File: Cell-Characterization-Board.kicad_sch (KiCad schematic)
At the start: 1 part, among them U1 ESP32-S3-WROOM-1

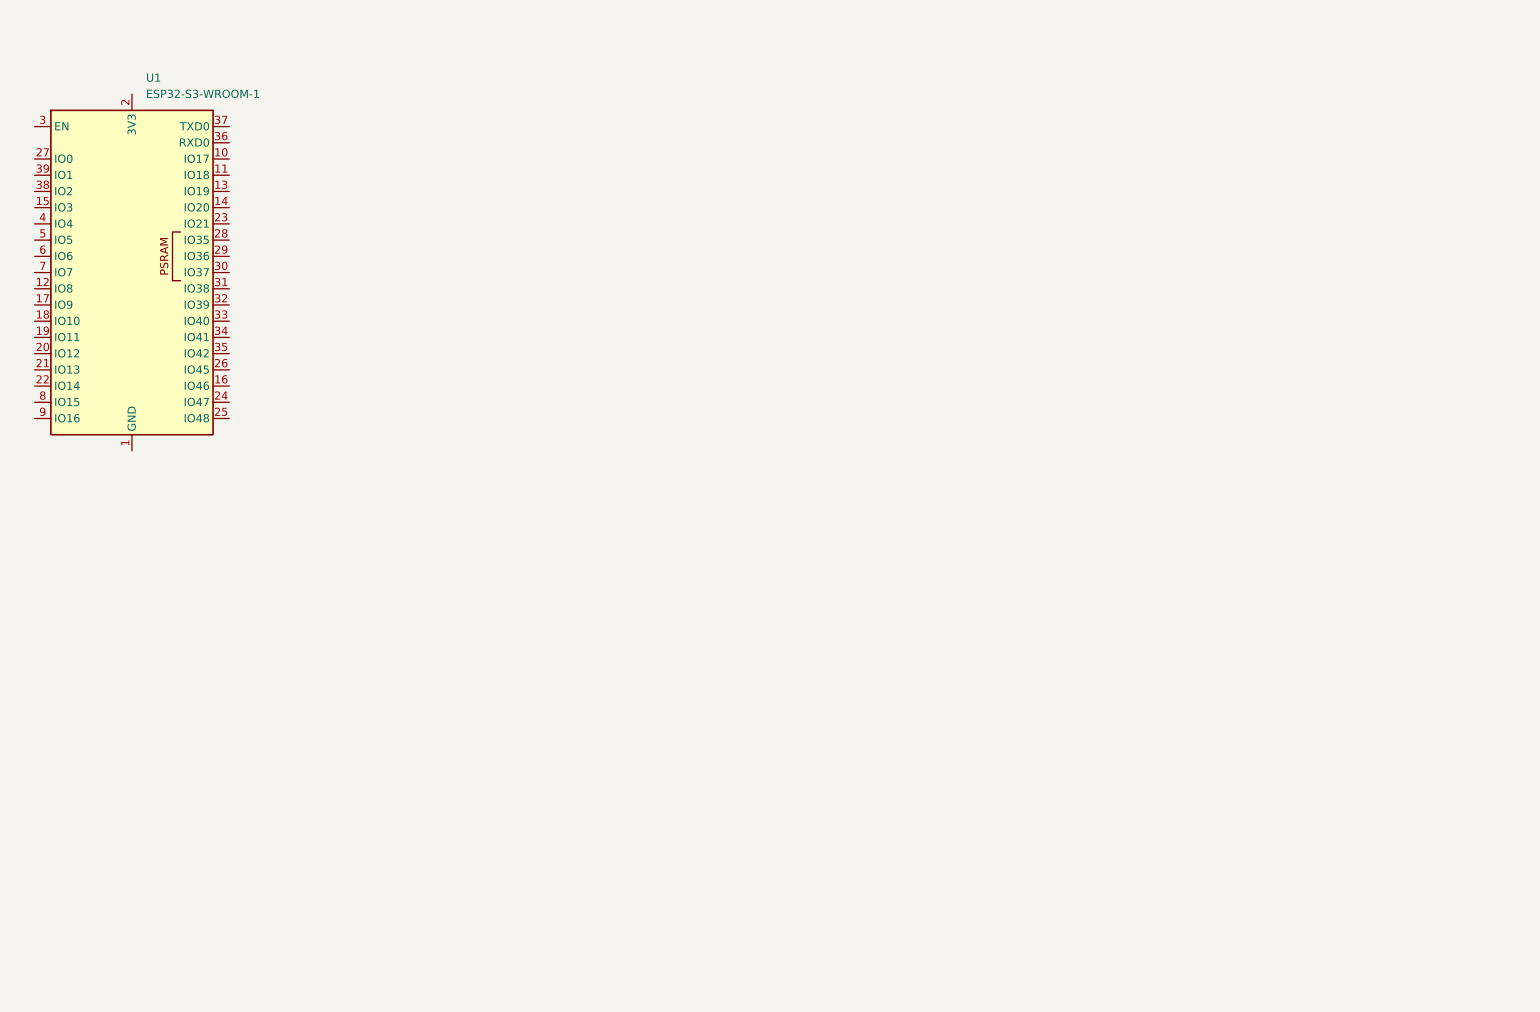
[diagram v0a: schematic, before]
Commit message: 🤪
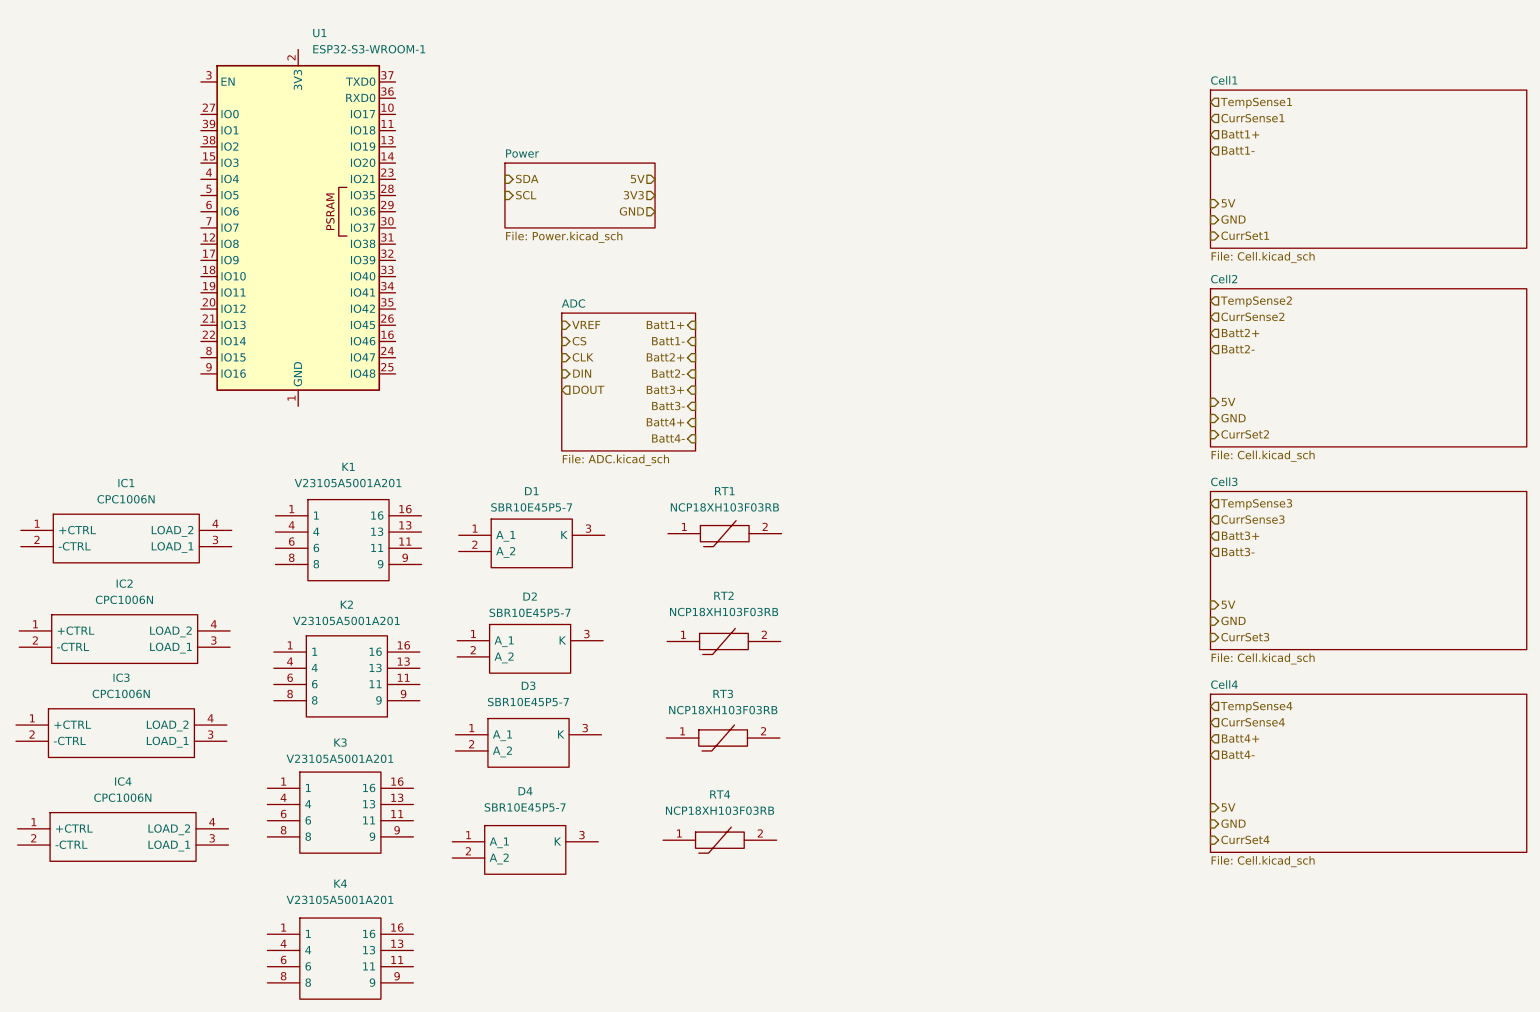
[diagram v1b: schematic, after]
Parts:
- added D1, D2, D3, D4: SBR10E45P5-7, SBR10E45P57, symbol SBR10E45P5-7:SBR10E45P5-7
- added IC1, IC2, IC3, IC4: CPC1006N, SOP254P610X216-4N, symbol CPC1006N:CPC1006N
- added K1, K2, K3, K4: V23105A5001A201, V23105A5001A201, symbol V23105A5001A201:V23105A5001A201
- added RT1, RT2, RT3, RT4: NCP18XH103F03RB, THRMC1608X95N, symbol NCP18XH103F03RB:NCP18XH103F03RB
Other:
- added sheet ADC (ADC.kicad_sch)
- added sheet Cell1 (Cell.kicad_sch)
- added sheet Cell2 (Cell.kicad_sch)
- added sheet Cell3 (Cell.kicad_sch)
- added sheet Cell4 (Cell.kicad_sch)
- added sheet Power (Power.kicad_sch)
- moved on the sheet: U1

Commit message: Updated main schematic
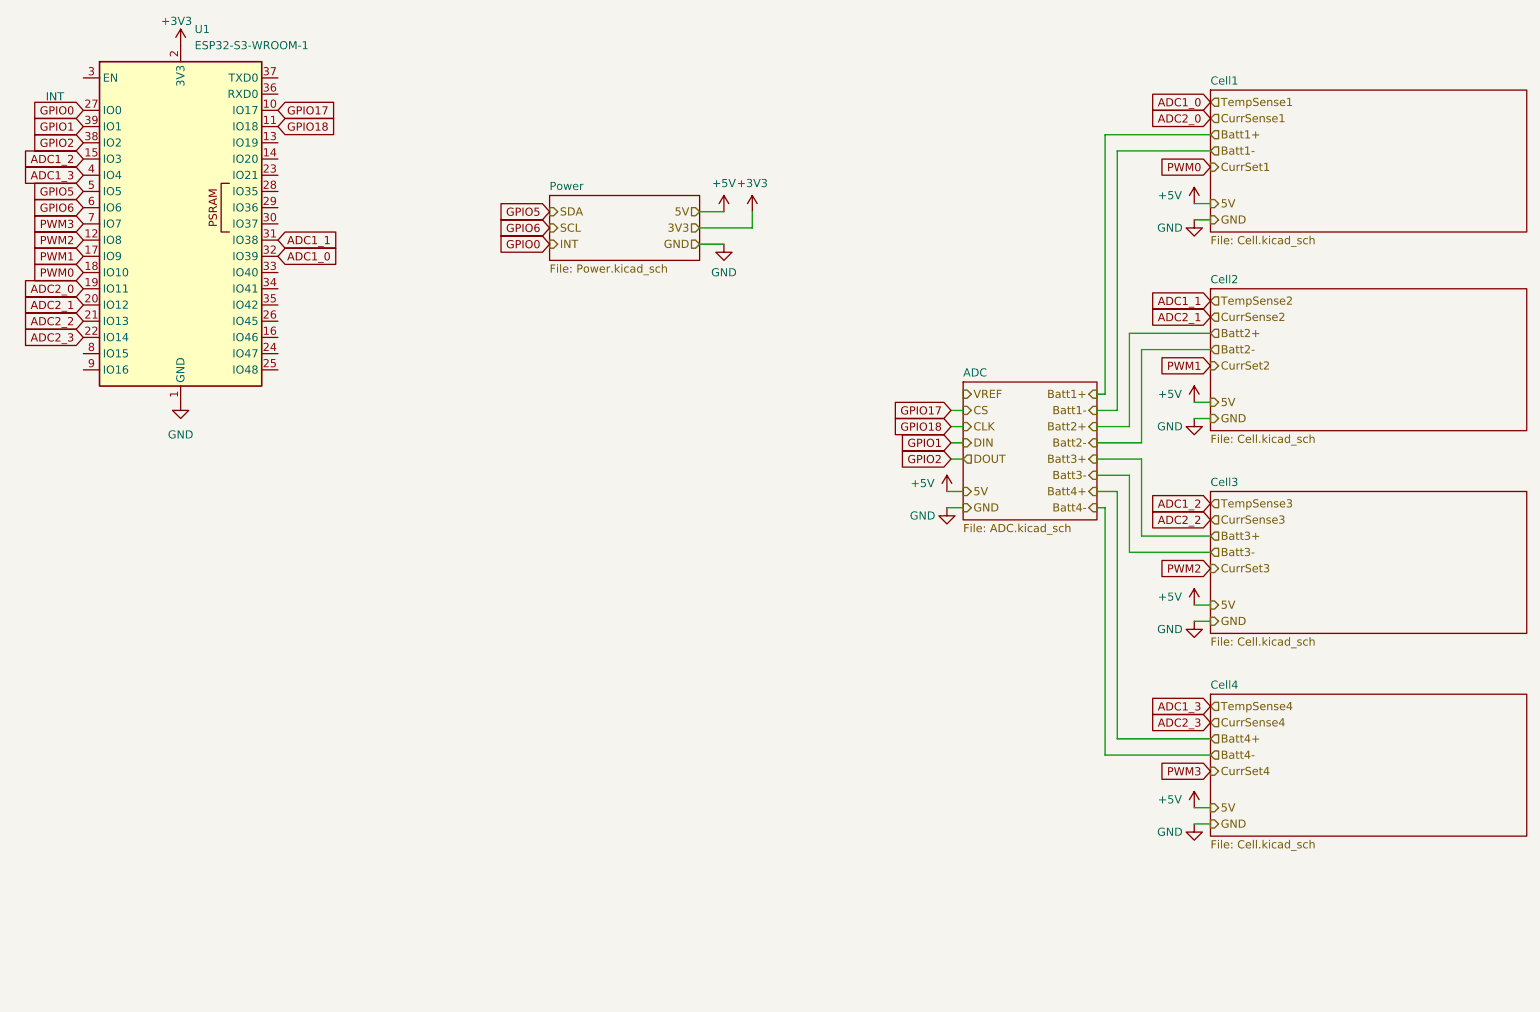
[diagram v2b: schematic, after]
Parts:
- removed D1, D2, D3, D4: SBR10E45P5-7, SBR10E45P57, symbol SBR10E45P5-7:SBR10E45P5-7
- removed IC1, IC2, IC3, IC4: CPC1006N, SOP254P610X216-4N, symbol CPC1006N:CPC1006N
- removed K1, K2, K3, K4: V23105A5001A201, V23105A5001A201, symbol V23105A5001A201:V23105A5001A201
- removed RT1, RT2, RT3, RT4: NCP18XH103F03RB, THRMC1608X95N, symbol NCP18XH103F03RB:NCP18XH103F03RB
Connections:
- net GND: now also U1.1 (GND), U1.40 (GND), U1.41 (GND)
- net GPIO17: now reaches U1.10 (IO17)
- net GPIO18: now reaches U1.11 (IO18)
- net PWM2: now reaches U1.12 (IO8)
- net ADC1_2: now reaches U1.15 (IO3)
- net PWM1: now reaches U1.17 (IO9)
- net PWM0: now reaches U1.18 (IO10)
- net ADC2_0: now reaches U1.19 (IO11)
- net +3V3: now reaches U1.2 (3V3)
- net ADC2_1: now reaches U1.20 (IO12)
- net ADC2_2: now reaches U1.21 (IO13)
- net ADC2_3: now reaches U1.22 (IO14)
- net GPIO0: now reaches U1.27 (IO0)
- net ADC1_1: now reaches U1.31 (IO38)
- net ADC1_0: now reaches U1.32 (IO39)
- net GPIO2: now reaches U1.38 (IO2)
- net GPIO1: now reaches U1.39 (IO1)
- net ADC1_3: now reaches U1.4 (IO4)
- net GPIO5: now reaches U1.5 (IO5)
- net GPIO6: now reaches U1.6 (IO6)
- net PWM3: now reaches U1.7 (IO7)
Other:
- note added: "INT"
- moved on the sheet: U1
